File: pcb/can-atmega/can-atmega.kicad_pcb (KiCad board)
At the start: 2 copper layers, 37 x 48 mm, 29 parts, among them J1 Screw_Terminal_01x05, J3 Conn_02x03_Odd_Even, J4 Connector_female, U1 LM1117-5.0, U2 TJA1051T, U3 MCP2515-xSO, U4 ATmega328P-A, X1 16MHz, X2 16MHz

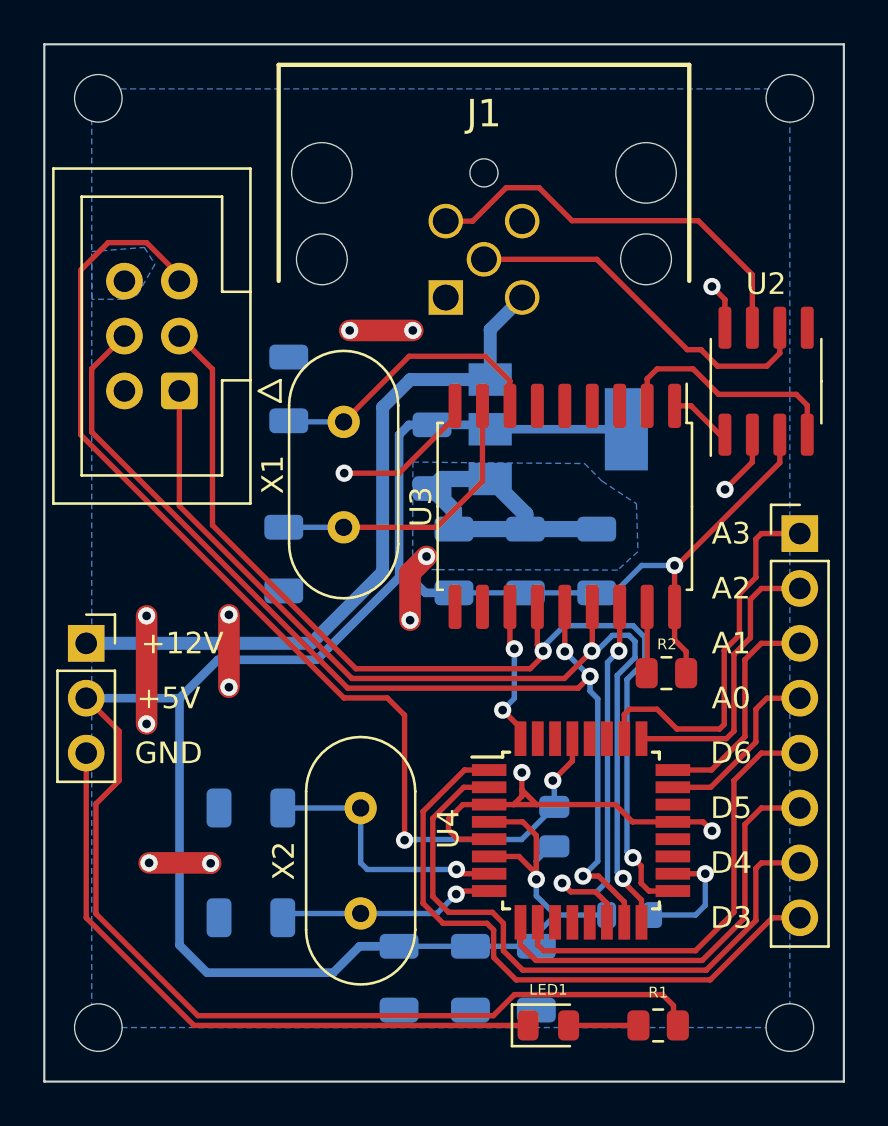
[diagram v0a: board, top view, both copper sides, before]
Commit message: pcb update
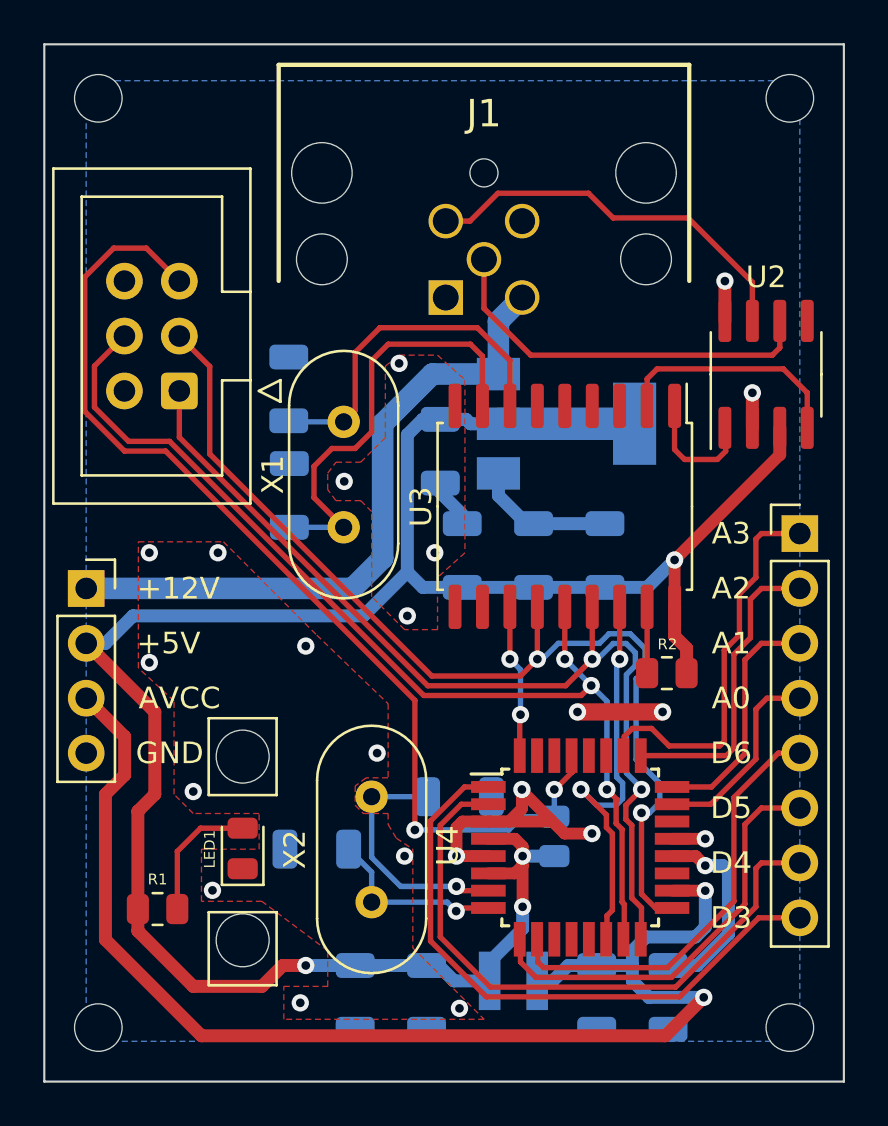
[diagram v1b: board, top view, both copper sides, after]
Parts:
- added C12: 22PF, Capacitor_SMD:C_1206_3216Metric, B.Cu at (152.9, 106.0)
- C10: value 22PF -> 0.1uF
- C7: value 0.1uF -> 10uF/16V
- C8: value 10uF/16V -> 0.1uF
- J4: value Connector_female -> Connector_female_4x8; footprint CAN_ATmega:Connector_female -> CAN_ATmega:Connector_female_4x8
- L1: footprint Inductor_SMD:L_0805_2012Metric -> Inductor_SMD:L_Neosid_SMS-ME3010
- LED1: footprint LED_SMD:LED_0805_2012Metric -> led_tube_MEN_12711000:led_tube_MEN_12711000
- moved R1 23.8 mm to (145.5, 108.8), turned to 0 degrees
- moved C10 21.2 mm to (169.2, 112.9), turned to 90 degrees
- moved LED1 16.3 mm to (149.5, 106.0), turned to 90 degrees
- moved C11 11.2 mm to (159.5, 103.6)
- moved C9 9.19 mm to (165.9, 112.9), turned to 90 degrees
- moved L1 6.18 mm to (162.0, 112.1)
- moved C7 5.41 mm to (154.7, 112.9)
- moved C8 5.16 mm to (158.0, 112.9)
- moved C5 2.96 mm to (151.6, 89.7), turned to -90 degrees
- moved J4 1.27 mm to (158.8, 99.1)
- moved U4 0.78 mm to (165.1, 106.0)
- moved X2 0.73 mm to (155.4, 103.6)
- moved C1 0.46 mm to (158.6, 87.6)
- moved U1 0.46 mm to (164.5, 86.4)
- moved C2 0.46 mm to (159.6, 92.5)
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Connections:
- C10 pad 1: /U4_OSC_1 -> GND
- C10 pad 2: GND -> /AREF
- C11 pad 1: GND -> /U4_OSC_1
- C11 pad 2: /U4_OSC_2 -> GND
- C9 pad 1: +5V -> GND
- C9 pad 2: GND -> AVCC
- J4 pad 10: U4_A2 -> U4_A1
- J4 pad 11: U4_A3 -> U4_A2
- J4 pad 3: GND -> AVCC
- J4 pad 4: U4_D3 -> GND
- J4 pad 5: U4_D4 -> U4_D3
- J4 pad 6: U4_D5 -> U4_D4
- J4 pad 7: U4_D6 -> U4_D5
- J4 pad 8: U4_A0 -> U4_D6
- J4 pad 9: U4_A1 -> U4_A0
- L1 pad 2: /AVCC -> AVCC
- U1 pad 4: (no net) -> +5V
- U4 pad 18: /AVCC -> AVCC
- U4 pad 20: unconnected-(U4-Pad20) -> /AREF
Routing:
- net GND: track 92.4 -> 30.9 mm, vias 15 -> 22
- net AVCC: track 0.00 -> 59.3 mm, vias 0 -> 2
- net +5V: track 147.0 -> 105.4 mm, vias 2 -> 4
- net /AREF: track 0.00 -> 9.21 mm, vias 0 -> 1
- net /U3_OSC_1: track 13.6 -> 20.5 mm
- net /AVCC: track 5.58 -> 0.00 mm, vias 1 -> 0
- net /U3_OSC_2: track 13.1 -> 16.3 mm
- net /U2_U3_TXD: track 2.88 -> 5.83 mm
- net /LED1: track 3.23 -> 6.14 mm
- net U4_RST: track 50.9 -> 48.4 mm
- net +12V: track 32.6 -> 30.8 mm
- net /U4_OSC_2: track 10.1 -> 8.56 mm
- net CAN_L: track 17.2 -> 18.2 mm
- net U4_D13_SCK: track 49.2 -> 48.2 mm
- net U4_D11_MOSI: track 50.0 -> 49.1 mm
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- added copper zone on F.Cu, net GND
